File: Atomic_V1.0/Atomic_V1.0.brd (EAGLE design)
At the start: 20 x 44 mm, 14 parts, among them U4 TLE9250VSJ, X1 S4P-VH

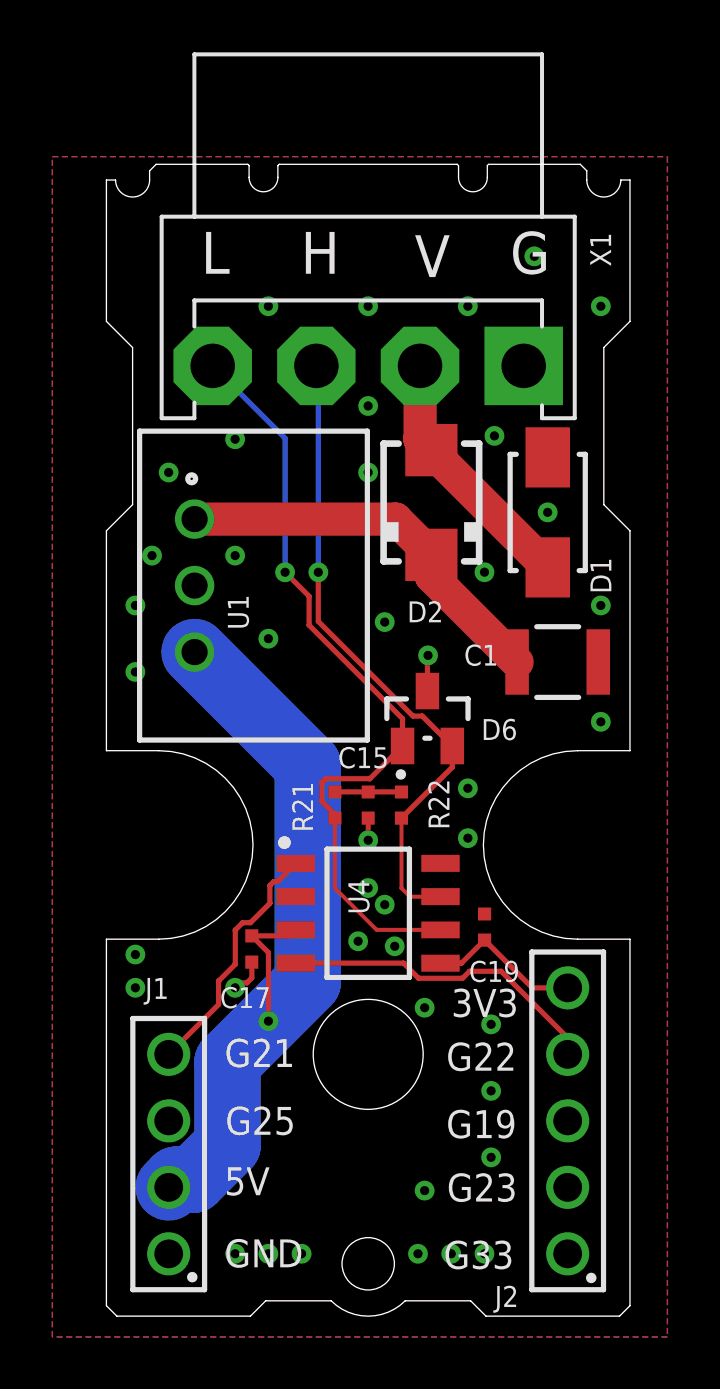
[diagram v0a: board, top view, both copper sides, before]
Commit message: collission avoid.
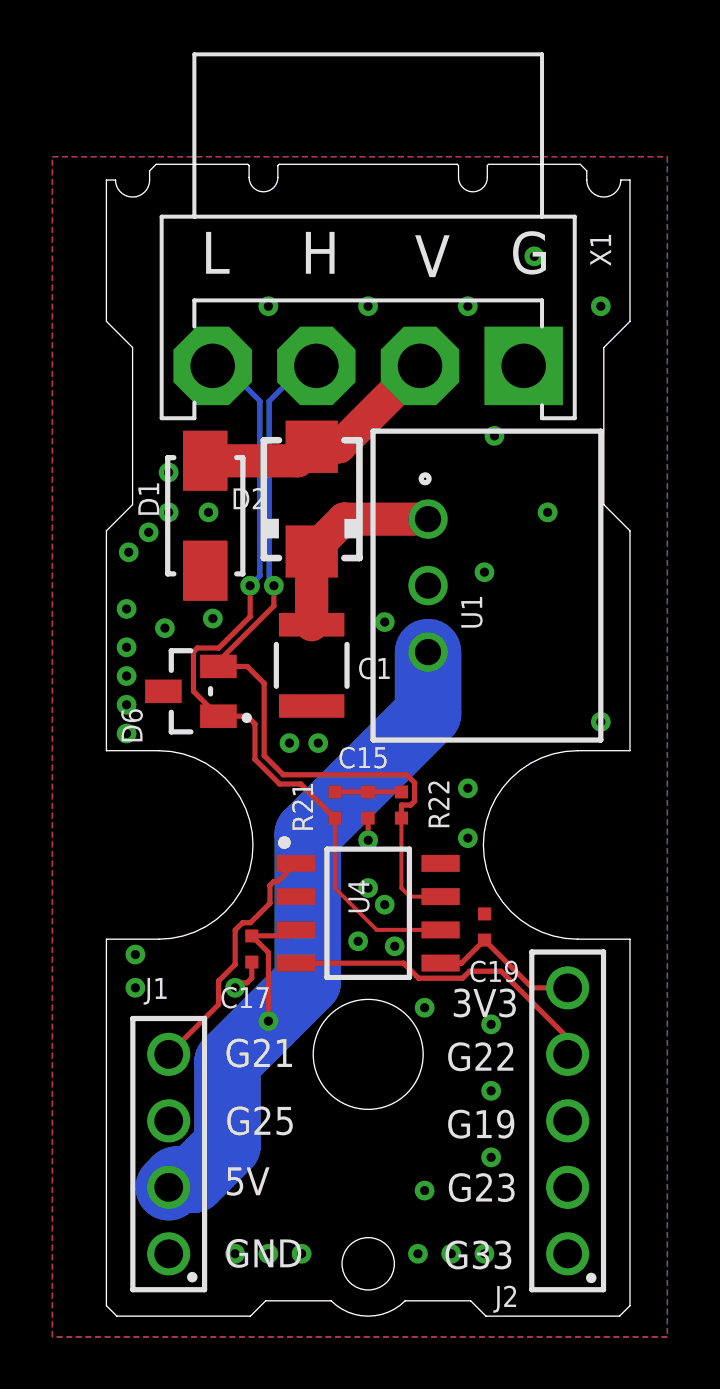
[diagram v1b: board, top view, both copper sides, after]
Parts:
- moved D1 13.1 mm to (1.40, 28.2), turned to 90 degrees
- moved C1 9.40 mm to (5.46, 22.5), turned to 90 degrees
- moved D6 9.09 mm to (0.85, 21.5), turned to 180 degrees
- moved U1 8.92 mm to (9.91, 25.5)
- moved D2 4.57 mm to (5.46, 28.8)
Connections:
- net CAN_H renamed CAN_P
- net CAN_L renamed CAN_N
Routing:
- net N$1: track 15.1 -> 7.76 mm
- net CAN_P: track 24.7 -> 30.5 mm
- net GND: track 3.62 -> 2.24 mm, vias 42 -> 45
- net +12V: track 10.3 -> 9.70 mm

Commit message: made PDF
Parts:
- C1: value 22µF -> 47uF
- D2: value S1ML -> SS12L R3
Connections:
- net CAN_N renamed CAN_L
- net CAN_P renamed CAN_H
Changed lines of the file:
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@@
 <attribute name="VCLAMP" value="42.1V" x="1.397" y="28.194" size="1.778" layer="27" rot="R90" display="off"/>
 </element>
-<element name="D2" library="fliegl-elektronik" package="SMA" value="S1ML" x="5.461" y="28.829" smashed="yes" rot="R90">
+<element name="D2" library="fliegl-elektronik" package="SMA" value="SS12L R3" x="5.461" y="28.829" smashed="yes" rot="R90">
 <attribute name="ARTIKEL_NR" value="505165" x="5.461" y="28.829" size="1.778" layer="27" rot="R90" display="off"/>
 <attribute name="NAME" x="3.766" y="29.242" size="0.8" layer="25" font="vector" ratio="10" rot="R180"/>
@@
 <attribute name="VALUE" x="8.326" y="27.095" size="1.27" layer="27" font="vector" ratio="10" rot="R90"/>
 </element>
-<element name="C1" library="Wurth_Capacitors_WCAP-CSGP" library_urn="urn:adsk.eagle:library:18488985" package="WCAP-CSGP_1210_H2.5" package3d_urn="urn:adsk.eagle:package:18489097/2" value="22µF" x="5.461" y="22.479" smashed="yes" rot="R90">
+<element name="C1" library="Wurth_Capacitors_WCAP-CSGP" library_urn="urn:adsk.eagle:library:18488985" package="WCAP-CSGP_1210_H2.5" package3d_urn="urn:adsk.eagle:package:18489097/2" value="47uF" x="5.461" y="22.479" smashed="yes" rot="R90">
 <attribute name="CERAMIC-TYPE" value="X5R Class II" x="5.461" y="22.479" size="1.778" layer="27" rot="R90" display="off"/>
 <attribute name="DATASHEET-URL" value="https://www.we-online.com/catalog/datasheet/885012109014.pdf" x="5.461" y="22.479" size="1.778" layer="27" rot="R90" display="off"/>
@@
 <wire x1="12.7" y1="10.795" x2="15.24" y2="8.255" width="0.2" layer="1"/>
 </signal>
-<signal name="CAN_P">
+<signal name="CAN_H">
 <contactref element="R22" pad="2"/>
 <contactref element="U4" pad="7"/>
@@
 <wire x1="9.09195" y1="18.3" x2="4.3784" y2="18.3" width="0.2" layer="1"/>
 </signal>
-<signal name="CAN_N">
+<signal name="CAN_L">
 <contactref element="R21" pad="1"/>
 <contactref element="U4" pad="6"/>
